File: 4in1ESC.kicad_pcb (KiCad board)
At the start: 6 copper layers, 31.2 x 33 mm, 179 parts, among them J1 SM08B-SRSS-TB, Q1 DOY180N03T, Q10 DOY180N03T, Q11 DOY180N03T, Q12 DOY180N03T, Q13 DOY180N03T, Q14 DOY180N03T, Q15 DOY180N03T, Q16 DOY180N03T, Q17 DOY180N03T, Q18 DOY180N03T, Q19 DOY180N03T, Q2 DOY180N03T, Q20 DOY180N03T, Q21 DOY180N03T, Q22 DOY180N03T, Q23 DOY180N03T, Q24 DOY180N03T, Q3 DOY180N03T, Q4 DOY180N03T, Q5 DOY180N03T, Q6 DOY180N03T, Q7 DOY180N03T, Q8 DOY180N03T, Q9 DOY180N03T, U1 TLV76733DRVR, U10 AT32F421G8U7, U11 NSG2065Q, U12 INA186A3IDCKR, U13 LMR54406DBVR, U2 AT32F421G8U7, U3 NSG2065Q, U5 FTC160808S4R7MBCA, U6 AT32F421G8U7, U7 NSG2065Q, U8 AT32F421G8U7, U9 NSG2065Q

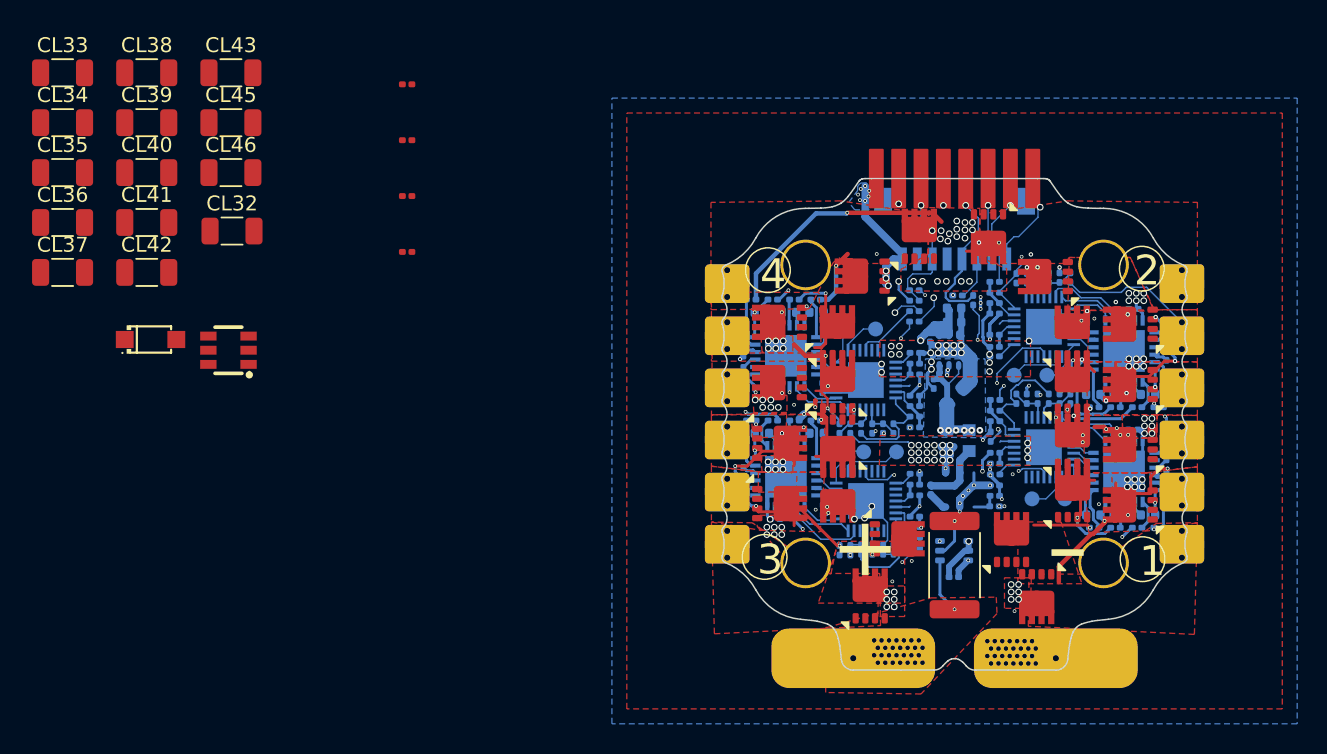
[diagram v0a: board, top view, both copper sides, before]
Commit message: alpha routing
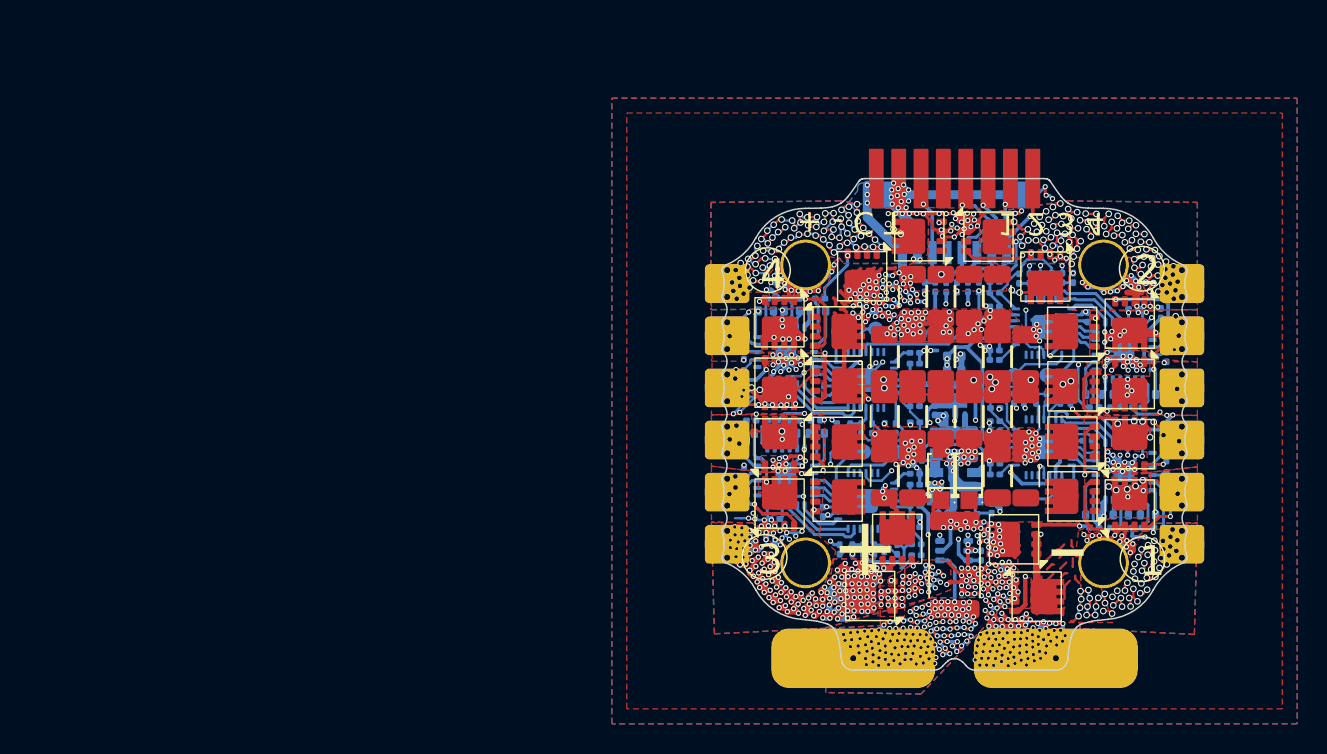
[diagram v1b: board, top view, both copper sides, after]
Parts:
- removed CL37, CL41: 10uF, Capacitor_SMD:C_1206_3216Metric
- added CL44: 10uF, Capacitor_SMD:C_1206_3216Metric, F.Cu at (80.8, 48.4)
- added CL47: 10uF, Capacitor_SMD:C_1206_3216Metric, F.Cu at (75.1, 48.4)
- added CL48: 10uF, Capacitor_SMD:C_1206_3216Metric, F.Cu at (73.2, 48.4)
- added CL49: 10uF, Capacitor_SMD:C_1206_3216Metric, F.Cu at (71.3, 48.4)
- added CL50: 10uF, Capacitor_SMD:C_1206_3216Metric, F.Cu at (71.3, 52.4)
- added CL51: 10uF, Capacitor_SMD:C_1206_3216Metric, F.Cu at (73.2, 52.4)
- added CL54: 10uF, Capacitor_SMD:C_1206_3216Metric, F.Cu at (78.9, 52.4)
- added CL55: 10uF, Capacitor_SMD:C_1206_3216Metric, F.Cu at (80.8, 52.4)
- added D2: SMF24A-T13, 4in1ESC:SOD-123FL_L2.7-W1.8-LS3.7-RD, F.Cu at (77.0, 52.2)
- C32, C33, C34, C35, C36, C37, C38, C39, C53, C59, C73, C83: footprint Capacitor_SMD:C_0402_1005Metric -> Capacitor_SMD:C_0402_WIDE
- R1, R10, R11, R12, R13, R14, R15, R16, R17, R18, R19, R2, R21, R22, R23, R24, R25, R26, R27, R28, R29, R3, R30, R31, R32, R33, R34, R35, R36, R37, R38, R39, R4, R40, R42, R43, R44, R45, R46, R47, R48, R49, R50, R51, R52, R53, R54, R55, R56, R57, R58, R6, R60, R61, R62, R63, R64, R65, R66, R67, R68, R69, R7, R70, R71, R72, R8, R9: footprint Capacitor_SMD:C_0201_0603Metric -> Resistor_SMD:R_0201_0603Metric
- R118, R73: footprint Capacitor_SMD:C_0201_0603Metric -> 4in1ESC:R_0201_0603Metric
- R74, R75, R76, R77, U13: moved to B.Cu
- U10, U2, U6, U8: footprint ESCLibrary:QFN-28_L4.0-W4.0-P0.40-TL-EP2.4 -> 4in1ESC:QFN-28_L4.0-W4.0-P0.40-TL-EP2.4
- U11, U3, U7, U9: footprint components:QFN-24_L4.0-W4.0-P0.50-TL-EP2.8 -> 4in1ESC:QFN-24_L4.0-W4.0-P0.50-TL-EP2.8
- U5: footprint components:IND-SMD_L1.6-W0.8_FTC160865SR47MBCA -> 4in1ESC:IND-SMD_L1.6-W0.8_FTC160865SR47MBCA
- moved CL33 64.5 mm to (78.9, 40.3), turned to -90 degrees
- moved CL34 62.0 mm to (77.0, 40.3), turned to -90 degrees
- moved CL35 59.5 mm to (75.1, 40.3), turned to -90 degrees
- moved CL42 57.4 mm to (78.9, 44.4), turned to 90 degrees
- moved CL36 57.3 mm to (73.2, 40.3), turned to -90 degrees
- moved CL43 56.7 mm to (80.8, 44.4), turned to 90 degrees
- moved CL45 55.1 mm to (78.9, 48.4), turned to -90 degrees
- moved CL40 54.7 mm to (75.1, 44.4), turned to 90 degrees
- moved D1 53.8 mm to (75.1, 52.3), turned to 90 degrees
- moved CL39 53.8 mm to (73.2, 44.4), turned to 90 degrees
- moved CL38 53.0 mm to (71.3, 44.4), turned to 90 degrees
- moved CL46 52.2 mm to (77.0, 48.4), turned to -90 degrees
- moved CL32 50.2 mm to (77.0, 44.4), turned to 90 degrees
- moved U13 49.6 mm to (76.0, 53.1)
- moved R74 41.5 mm to (78.7, 50.1), turned to 180 degrees
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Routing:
- net GND: track 73.6 -> 417.4 mm, vias 171 -> 460
- net +BATT: track 17.9 -> 111.8 mm, vias 20 -> 113
- net +10V: track 11.9 -> 84.5 mm, vias 10 -> 7
- net /ESC3/MotorA: track 15.0 -> 83.3 mm, vias 4 -> 144
- net /CSA+: track 3.69 -> 72.0 mm, vias 29 -> 140
- net /ESC2/MotorA: track 16.4 -> 80.3 mm, vias 3 -> 101
- net /ESC4/MotorA: track 19.7 -> 74.3 mm, vias 3 -> 85
- net /ESC1/MotorA: track 19.9 -> 71.9 mm, vias 4 -> 58
- net /ESC4/MotorC: track 9.95 -> 32.1 mm, vias 2 -> 15
- net /M4: track 25.0 -> 8.68 mm, vias 2 -> 1
- net /ESC1/MotorB: track 10.1 -> 25.5 mm, vias 3 -> 9
- net /ESC2/MotorC: track 14.1 -> 28.5 mm, vias 1 -> 12
- net /ESC2/MotorB: track 12.7 -> 23.3 mm, vias 2 -> 6
- net /ESC1/MotorC: track 14.7 -> 25.0 mm, vias 2 -> 9
- net /ESC4/MotorB: track 11.7 -> 20.0 mm, vias 2 -> 10
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- added copper zone on B.Cu, net /CSA+
- added copper zone on In1.Cu, net /CSA+
- added copper zone on In2.Cu, net /CSA+
- added copper zone on In3.Cu, net /CSA+
- added copper zone on In4.Cu, net /CSA+
- added copper zone on B.Cu, net /ESC1/MotorA
- added copper zone on In2.Cu, net /ESC1/MotorA
- added copper zone on In3.Cu, net /ESC1/MotorA
- added copper zone on B.Cu, net /ESC2/MotorA
- added copper zone on In2.Cu, net /ESC2/MotorA
- added copper zone on In3.Cu, net /ESC2/MotorA
- added copper zone on B.Cu, net /ESC3/MotorA
- added copper zone on In1.Cu, net /ESC3/MotorA
- added copper zone on In2.Cu, net /ESC3/MotorA
- added copper zone on In3.Cu, net /ESC3/MotorA
- added copper zone on In4.Cu, net /ESC3/MotorA
- added copper zone on B.Cu, net /ESC4/MotorA
- added copper zone on In2.Cu, net /ESC4/MotorA
- added copper zone on In3.Cu, net /ESC4/MotorA
- added copper zone on In2.Cu, net GND
- removed copper zone on B.Cu, net +10V
- removed copper zone on In2.Cu, net +10V
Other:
- board text added: "3-6S"
- board text added: "AM32"
- board text removed: "+ -C T 1 2 3 4"
- board text removed: "3-6S input"
- board text removed: "AM32 ESC"
- board text removed: "pin order:"
